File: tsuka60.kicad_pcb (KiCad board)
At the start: 2 copper layers, 285 x 95.1 mm, 179 parts, among them SW1 SW_Push, U1 ATmega32U4-AU, Y1 Resonator_Small

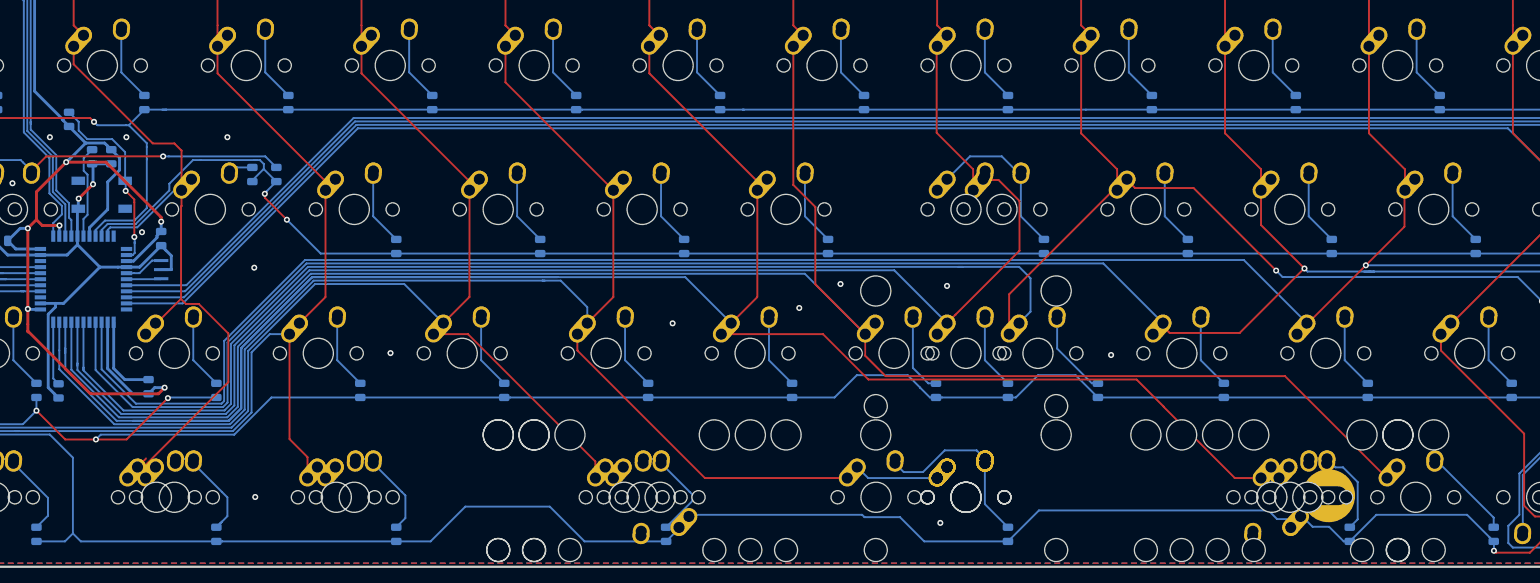
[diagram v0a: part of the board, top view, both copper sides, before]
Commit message: removed lots of compatibility
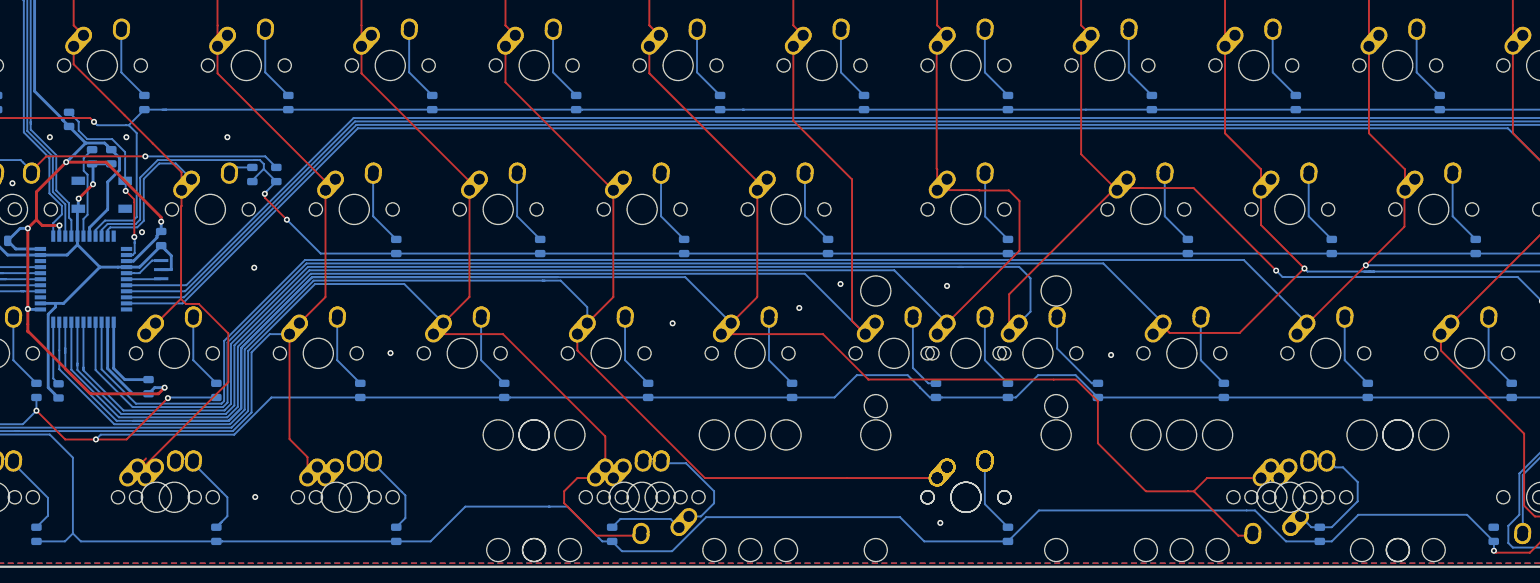
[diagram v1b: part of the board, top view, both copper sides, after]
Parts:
- removed MX37: LEGACY-H, MX_Alps_Hybrid:MX-1U-NoLED
- removed MX65-3: SPACE, MX_Alps_Hybrid:MX-6.25U-ReversedStabilizers-NoLED
- removed MX67-3: LEGACY-BOTTOM, MX_Alps_Hybrid:MX-1.25U-NoLED
- moved D64 7.14 mm to (190.5, 202.6)
- moved D38 4.76 mm to (242.9, 164.4)
- moved D66 3.97 mm to (284.2, 202.6)
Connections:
- MX38 pad 1: Net-(D38-Pad2) -> Col7
- MX38 pad 2: Col7 -> Net-(D38-Pad2)
- MX64-ALPS-1 pad 1: Col3 -> Net-(D64-Pad2)
- MX64-ALPS-1 pad 2: Net-(D64-Pad2) -> Col3
- MX66-ALPS-1 pad 1: Col5 -> Net-(D66-Pad2)
- MX66-ALPS-1 pad 2: Net-(D66-Pad2) -> Col5
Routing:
- net Col6: track 268.6 -> 190.0 mm
- net Col3: track 208.2 -> 230.7 mm
- net Col5: track 325.0 -> 340.1 mm
- net Net-(D65-Pad2): track 23.8 -> 9.73 mm
- net Net-(D64-Pad2): track 14.2 -> 26.6 mm
- net Net-(D67-Pad2): track 12.1 -> 0.00 mm
- net Net-(D38-Pad2): track 21.8 -> 12.1 mm
- net Col1: track 112.1 -> 118.3 mm
- net Net-(D66-Pad2): track 14.6 -> 20.3 mm
- net Row2: track 263.2 -> 265.9 mm
- net Col8: track 308.7 -> 310.7 mm
- net Row1: track 294.8 -> 293.7 mm
- net Col7: track 207.3 -> 208.5 mm
- net Row4: track 357.7 -> 358.7 mm
- net Col4: track 215.7 -> 216.4 mm
